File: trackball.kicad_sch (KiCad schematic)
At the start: 174 parts, among them J1 ZX-PM2.0-2-4PY, SW1 HX TC-5608-Y, SW2 HX TC-5608-Y, SW3 HX TC-5608-Y, SW4 HX TC-5608-Y, SW5 HX TC-5608-Y, SW6 HX TC-5608-Y, SW7 HX TC-5608-Y, SW8 HX TC-5608-Y, U1 SY8089A1AAC, U10 WS2812B, U11 WS2812B, U12 WS2812B, U13 WS2812B, U14 WS2812B, U15 WS2812B, U16 WS2812B, U17 WS2812B, U18 WS2812B, U19 WS2812B, U2 USB-TYPE-C-017, U20 WS2812B, U3 PMW3610, U4 PMW3610, U5 WS2812B, U6 WS2812B, U7 WS2812B, U8 WS2812B, U9 WS2812B, X1 XL7EL89CKI-111YLC-32M

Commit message: chore: checkpoint
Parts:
- R1, R10, R15, R16, R20, R21, R22, R23, R24, R27, R28, R3, R32, R33, R34, R37, R38, R39, R4, R40, R41, R42, R45, R48, R54, R55, R9: LCSC Part C364845 -> C273334
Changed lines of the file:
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@@
 			)
 		)
-		(property "LCSC Part" "C364845"
+		(property "LCSC Part" "C273334"
 			(at 207.01 308.61 0)
 			(effects
@@
 			)
 		)
-		(property "LCSC Part" "C364845"
+		(property "LCSC Part" "C273334"
 			(at 464.82 67.31 0)
 			(effects
@@
 			)
 		)
-		(property "LCSC Part" "C364845"
+		(property "LCSC Part" "C273334"
 			(at 288.29 83.82 0)
 			(effects
@@
 			)
 		)
-		(property "LCSC Part" "C364845"
+		(property "LCSC Part" "C273334"
 			(at 424.18 143.51 0)
 			(effects
@@
 			)
 		)
-		(property "LCSC Part" "C364845"
+		(property "LCSC Part" "C273334"
 			(at 223.52 290.83 0)
 			(effects
@@
 			)
 		)
-		(property "LCSC Part" "C364845"
+		(property "LCSC Part" "C273334"
 			(at 378.46 116.84 0)
 			(effects
@@
 			)
 		)
-		(property "LCSC Part" "C364845"
+		(property "LCSC Part" "C273334"
 			(at 299.72 83.82 0)
 			(effects
@@
 			)
 		)
-		(property "LCSC Part" "C364845"
+		(property "LCSC Part" "C273334"
 			(at 474.98 402.59 0)
 			(effects
@@
 			)
 		)
-		(property "LCSC Part" "C364845"
+		(property "LCSC Part" "C273334"
 			(at 464.82 46.99 0)
 			(effects
@@
 			)
 		)
-		(property "LCSC Part" "C364845"
+		(property "LCSC Part" "C273334"
 			(at 424.18 116.84 0)
 			(effects
@@
 			)
 		)
-		(property "LCSC Part" "C364845"
+		(property "LCSC Part" "C273334"
 			(at 474.98 411.48 0)
 			(effects
@@
 			)
 		)
-		(property "LCSC Part" "C364845"
+		(property "LCSC Part" "C273334"
 			(at 462.28 195.58 0)
 			(effects
@@
 			)
 		)
-		(property "LCSC Part" "C364845"
+		(property "LCSC Part" "C273334"
 			(at 485.14 100.33 0)
 			(effects
@@
 			)
 		)
-		(property "LCSC Part" "C364845"
+		(property "LCSC Part" "C273334"
 			(at 365.76 87.63 0)
 			(effects
@@
 			)
 		)
-		(property "LCSC Part" "C364845"
+		(property "LCSC Part" "C273334"
 			(at 462.28 128.27 0)
 			(effects
@@
 			)
 		)
-		(property "LCSC Part" "C364845"
+		(property "LCSC Part" "C273334"
 			(at 207.01 290.83 0)
 			(effects
@@
 			)
 		)
-		(property "LCSC Part" "C364845"
+		(property "LCSC Part" "C273334"
 			(at 491.49 240.03 0)
 			(effects
@@
 			)
 		)
-		(property "LCSC Part" "C364845"
+		(property "LCSC Part" "C273334"
 			(at 444.5 153.67 0)
 			(effects
@@
 			)
 		)
-		(property "LCSC Part" "C364845"
+		(property "LCSC Part" "C273334"
 			(at 424.18 196.85 0)
 			(effects
@@
 			)
 		)
-		(property "LCSC Part" "C364845"
+		(property "LCSC Part" "C273334"
 			(at 491.49 172.72 0)
 			(effects
@@
 			)
 		)
-		(property "LCSC Part" "C364845"
+		(property "LCSC Part" "C273334"
 			(at 378.46 143.51 0)
 			(effects
@@
 			)
 		)
-		(property "LCSC Part" "C364845"
+		(property "LCSC Part" "C273334"
 			(at 223.52 308.61 0)
 			(effects
@@
 			)
 		)
-		(property "LCSC Part" "C364845"
+		(property "LCSC Part" "C273334"
 			(at 378.46 196.85 0)
 			(effects
@@
 			)
 		)
-		(property "LCSC Part" "C364845"
+		(property "LCSC Part" "C273334"
 			(at 424.18 170.18 0)
 			(effects
@@
 			)
 		)
-		(property "LCSC Part" "C364845"
+		(property "LCSC Part" "C273334"
 			(at 444.5 220.98 0)
 			(effects
@@
 			)
 		)
-		(property "LCSC Part" "C364845"
+		(property "LCSC Part" "C273334"
 			(at 464.82 57.15 0)
 			(effects
@@
 			)
 		)
-		(property "LCSC Part" "C364845"
+		(property "LCSC Part" "C273334"
 			(at 378.46 170.18 0)
 			(effects

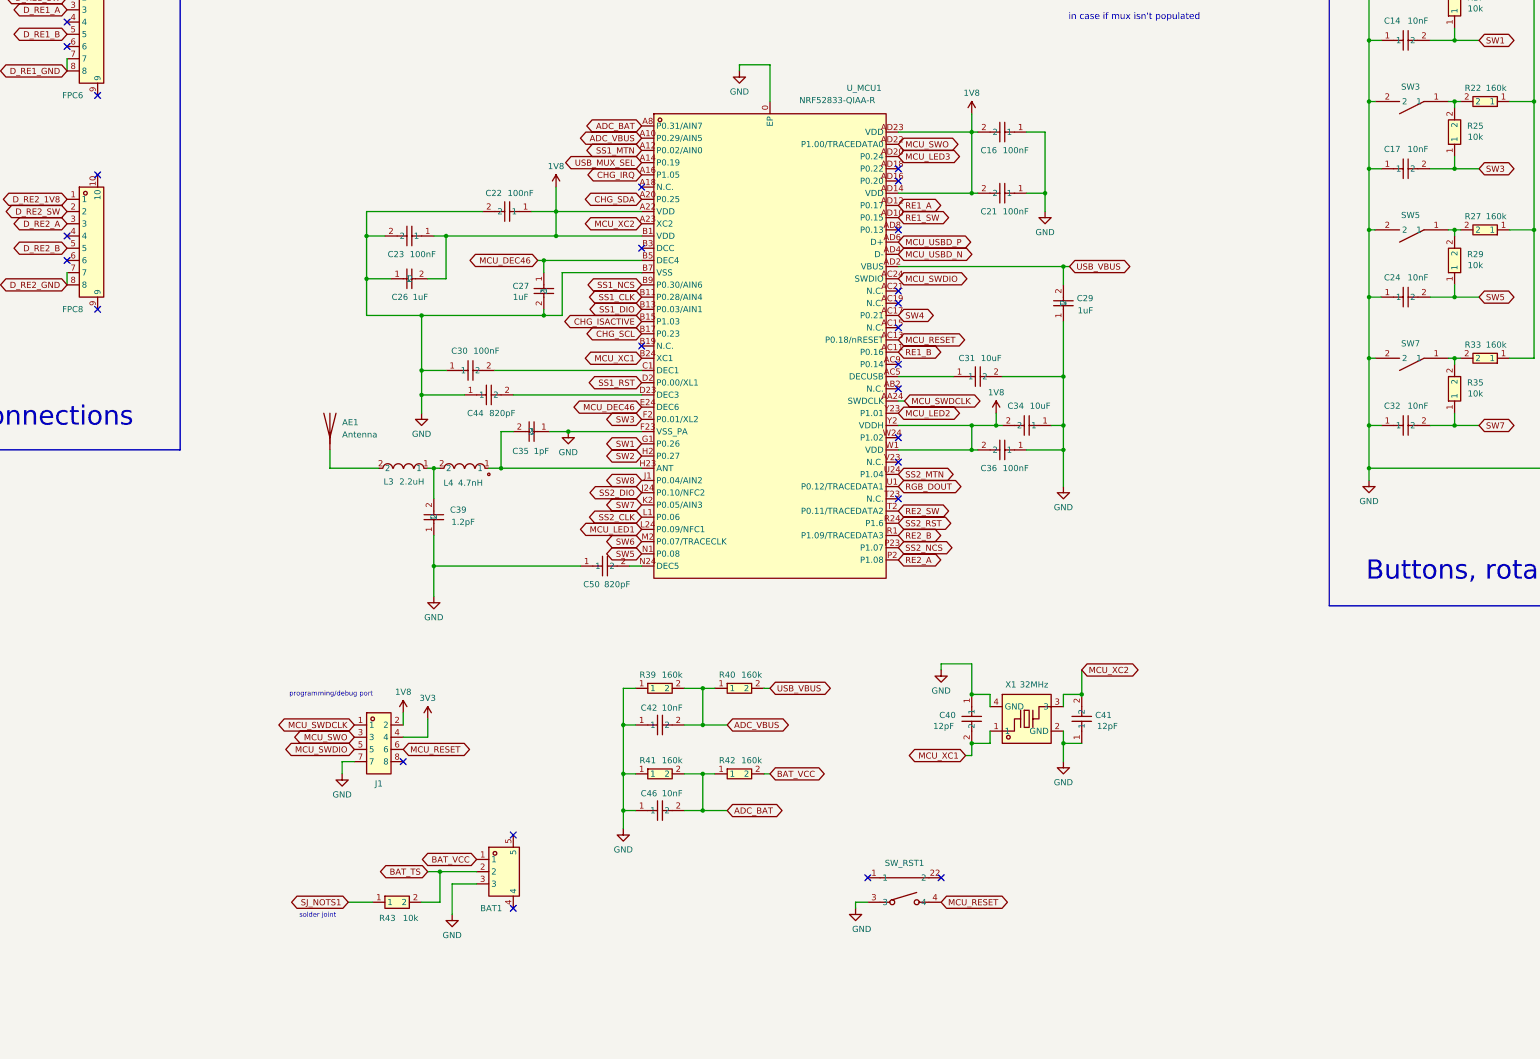
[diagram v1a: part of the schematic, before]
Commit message: chore: checkpoint
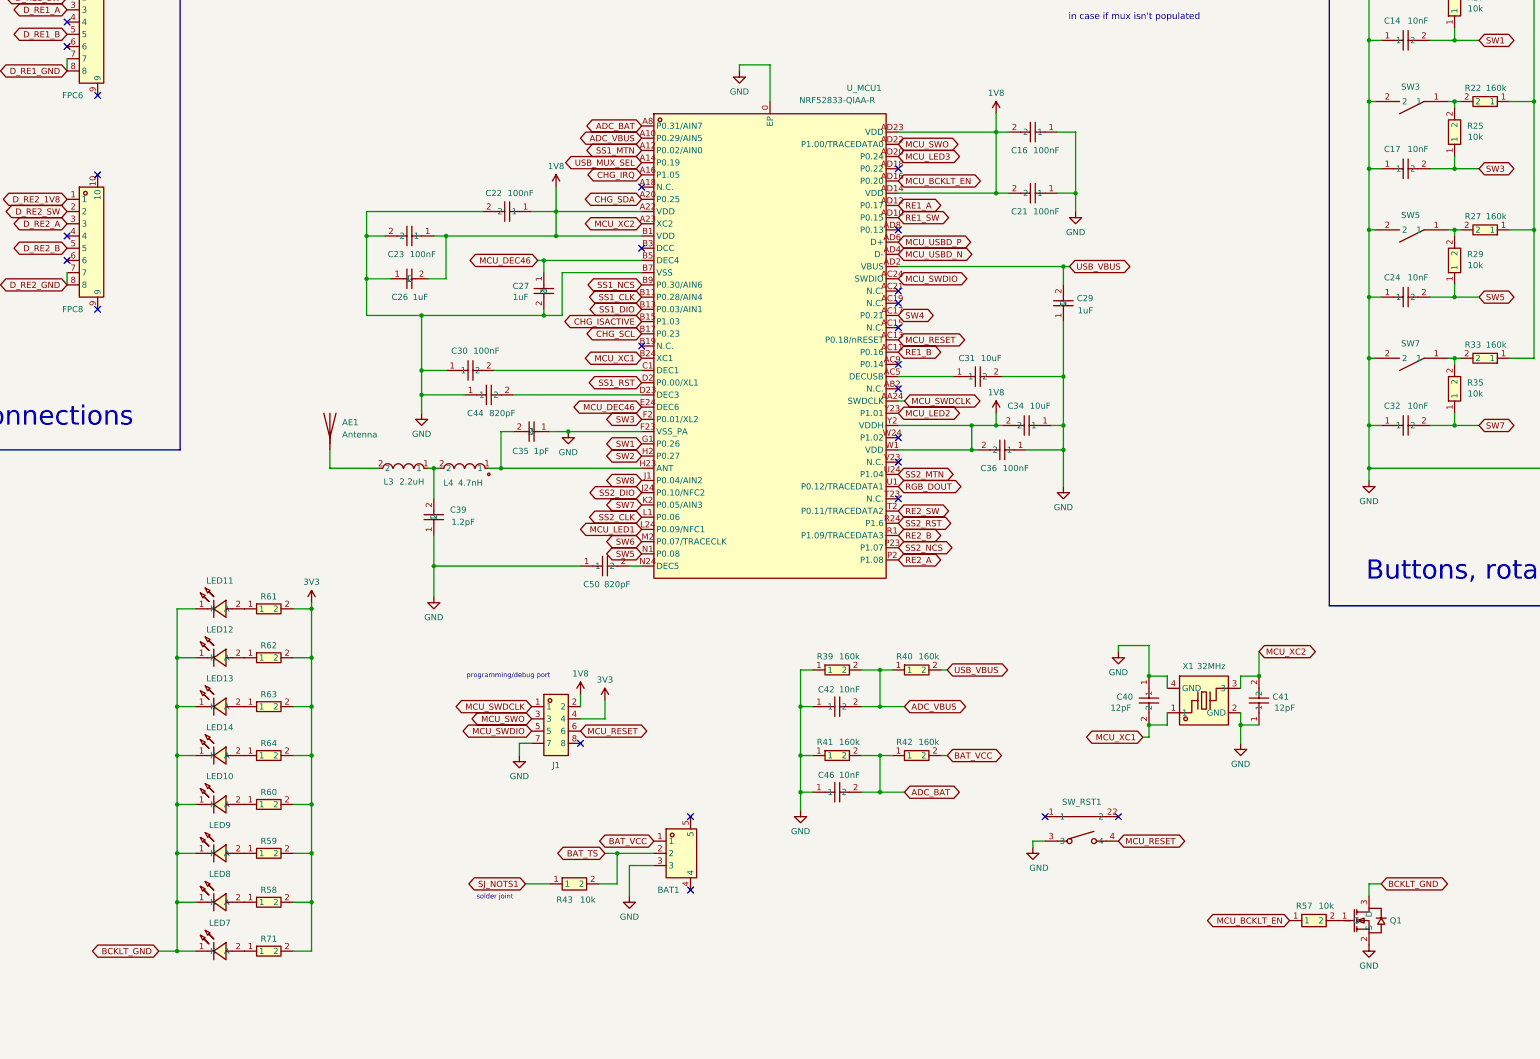
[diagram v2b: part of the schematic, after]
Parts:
- added LED10, LED11, LED12, LED13, LED14, LED7, LED8, LED9: SZYY0402W, easyeda2kicad:LED0402-RD_WHITE, symbol easyeda2kicad:SZYY0402W
- added Q1: SI2302_C2891732, easyeda2kicad:SOT-23-3_L2.9-W1.3-P1.90-LS2.4-BR, symbol easyeda2kicad:SI2302_C2891732
- added R57: FRC0402F1002TS, easyeda2kicad:R0402, symbol easyeda2kicad:FRC0402F1002TS
- added R58, R59, R60, R61, R62, R63, R64, R71: RT0402BRE0750RL, easyeda2kicad:R0402, symbol easyeda2kicad:RT0402BRE0750RL
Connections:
- net 3V3: now also R58.2, R59.2, R60.2, R61.2, R62.2, R63.2, R64.2, R71.2
- net GND: now also Q1.2 (S)
- net MCU_BCKLT_EN: now reaches U_MCU1.AD16 (P0.20)
- net MCU_BCKLT_EN: now also R57.1
- new net: LED13.2 (A), R63.1
- new net: LED7.2 (A), R71.1
- new net: Q1.1 (G), R57.2
- new net: LED12.2 (A), R62.1
- new net: LED9.2 (A), R59.1
- new net: LED11.2 (A), R61.1
- new net: LED14.2 (A), R64.1
- new net: LED10.2 (A), R60.1
- new net: LED8.2 (A), R58.1
- new net BCKLT_GND: LED10.1 (K), LED11.1 (K), LED12.1 (K), LED13.1 (K), LED14.1 (K), LED7.1 (K), LED8.1 (K), LED9.1 (K), Q1.3 (D)
- no-connect marks 53 -> 52
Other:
- moved on the sheet: BAT1, C16, C21, C40, C41, C42, C46, J1, R39, R40, R41, R42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

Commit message: chore: checkpoint
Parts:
- added LED15: PD15-22C/TR8, easyeda2kicad:SENSOR-SMD_PD15-22C-TR8, symbol easyeda2kicad:PD15-22C_TR8
- added R65, R66: FRC0402F1002TS, easyeda2kicad:R0402, symbol easyeda2kicad:FRC0402F1002TS
- added U21: ANT3216LL00R2400A, easyeda2kicad:ANT-SMD_L3.2-W1.6, symbol easyeda2kicad:ANT3216LL00R2400A
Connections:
- net 3V3: now also LED15.1 (C), LED15.4 (C)
- net CHG_ADC: now also LED15.2 (A), LED15.3 (A), R65.2
- net GND: now also R66.1
- new net: R65.1, R66.2
- no-connect marks 52 -> 54
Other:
- note added: "alternative antenna? 5dBi stated"
- moved on the sheet: BAT1, J1, LED10, LED11, LED12, LED13, LED14, LED7, LED8, LED9, R43, R58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
